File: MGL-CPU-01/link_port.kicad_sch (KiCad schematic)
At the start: 9 parts, among them P3 GameBoy_LinkPort

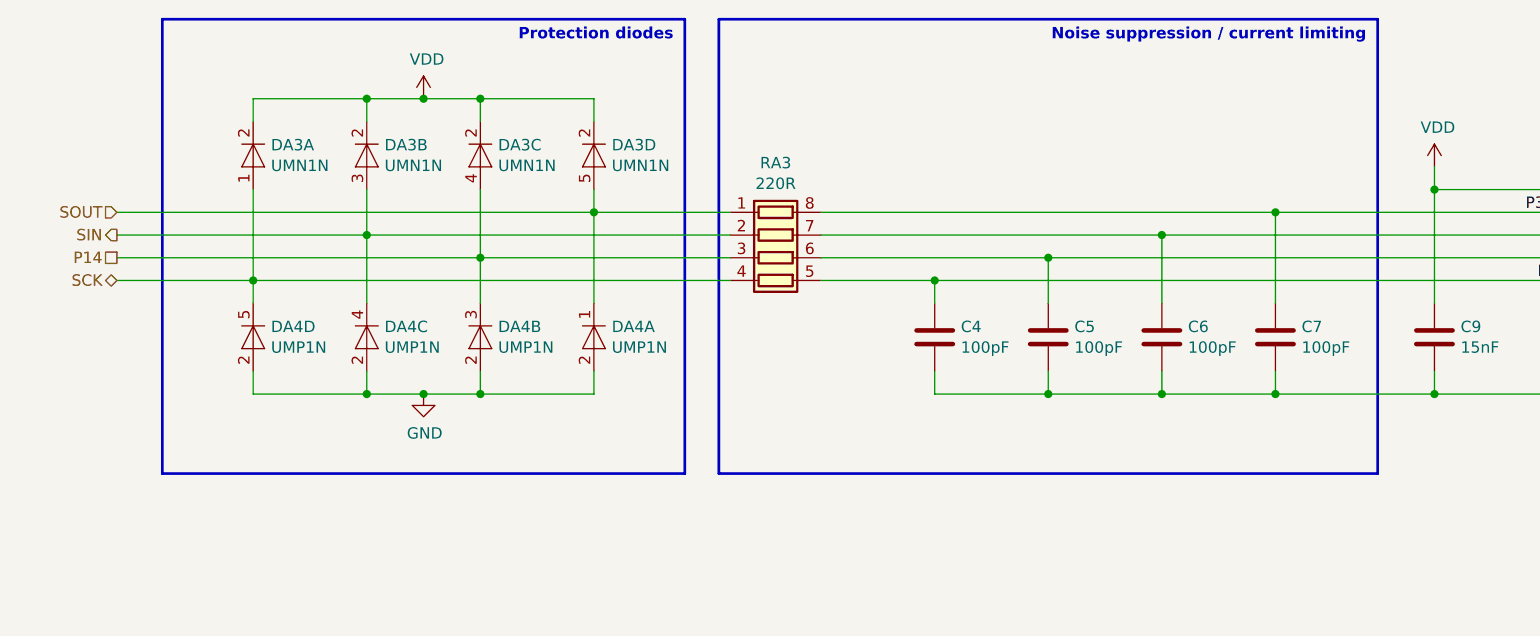
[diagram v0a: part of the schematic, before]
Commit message: Update to latest KiCad
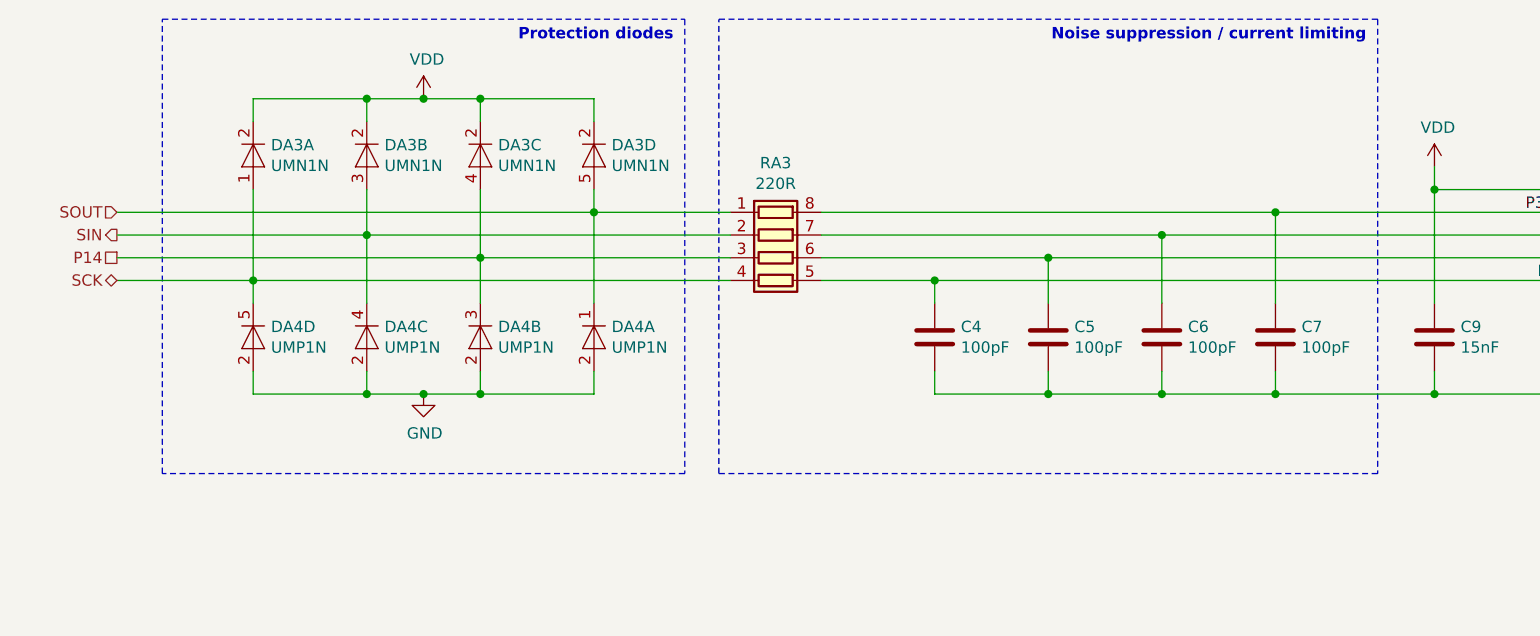
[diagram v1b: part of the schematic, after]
